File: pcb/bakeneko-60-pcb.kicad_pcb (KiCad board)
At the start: 2 copper layers, 284.8 x 106.7 mm, 149 parts, among them J1 JST SH 4-pin, SW1 Reset, U1 SRV05-4, U2 ATmega32U4-AU, Y1 16MHz

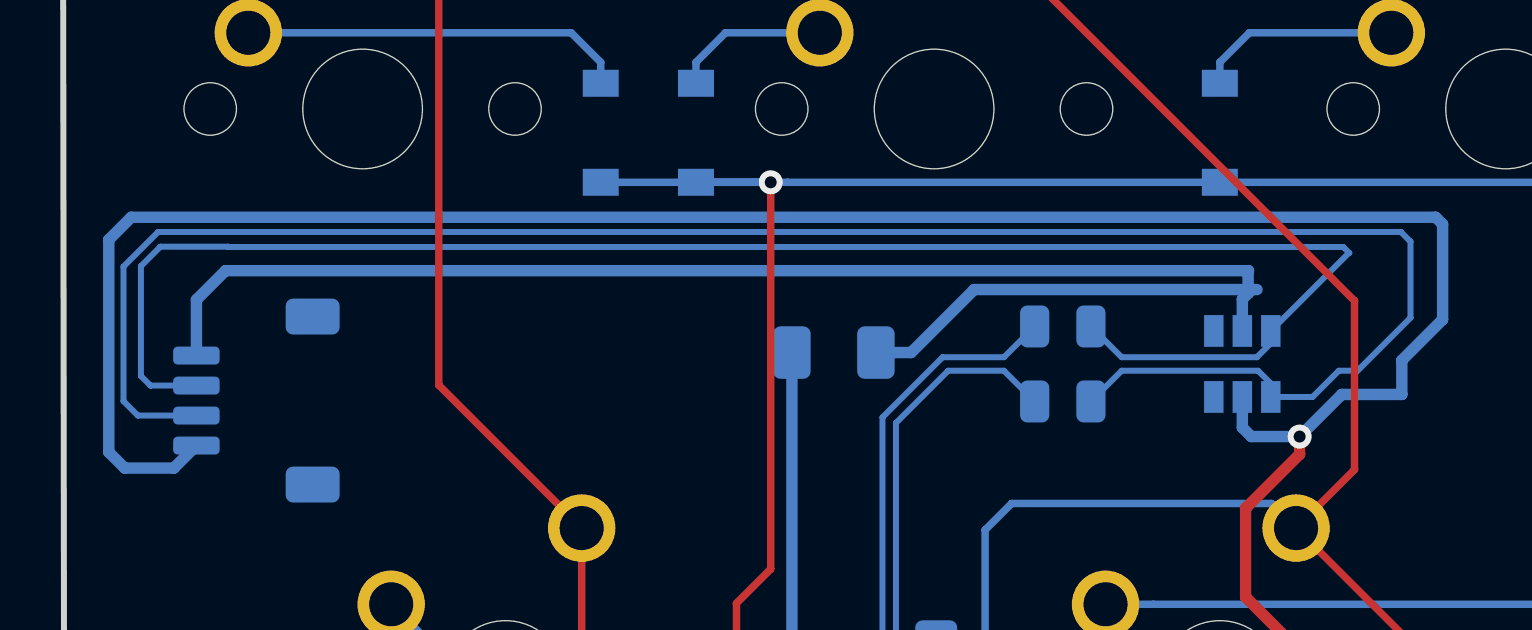
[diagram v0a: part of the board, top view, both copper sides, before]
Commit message: cleanup tracks
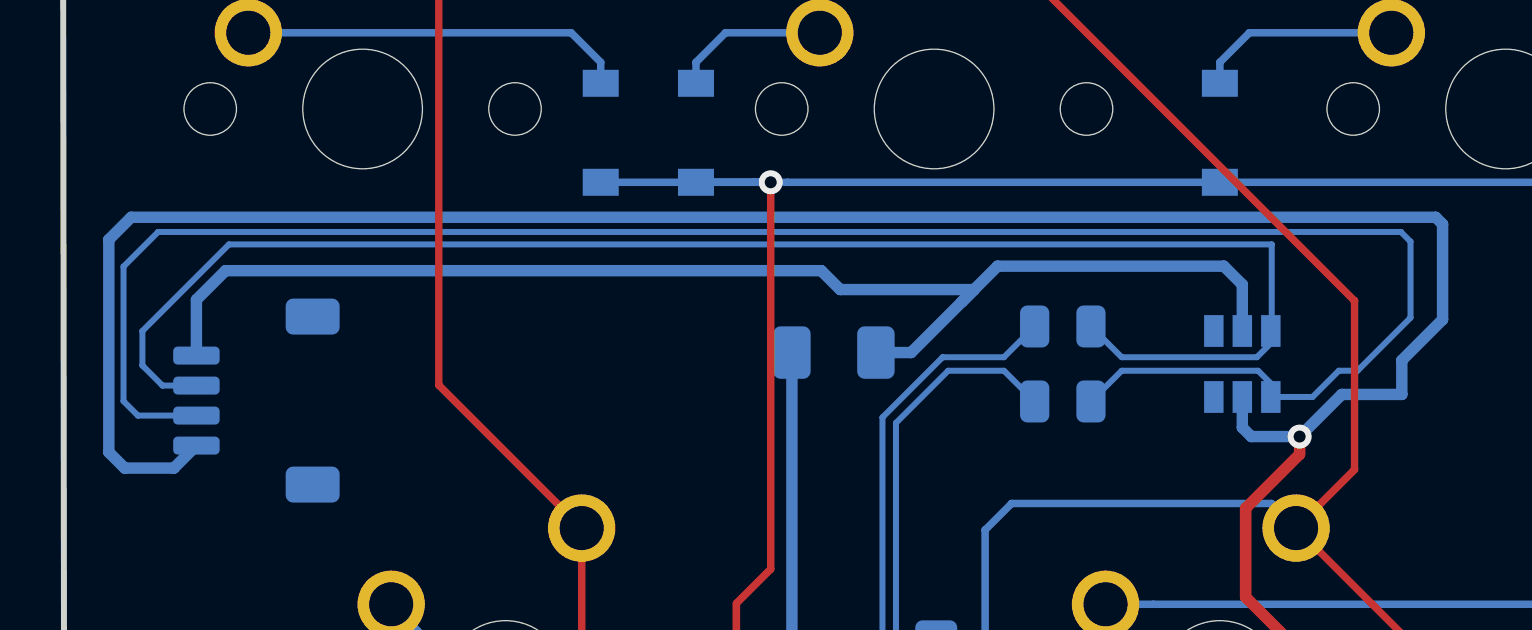
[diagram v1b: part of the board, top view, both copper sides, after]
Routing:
- net VBUS: track 53.2 -> 44.2 mm
- net D-: track 57.0 -> 52.0 mm
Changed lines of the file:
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@@
   (segment (start 262.34625 82.66) (end 261.3625 83.64375) (width 0.25) (layer "B.Cu") (net 71))
   (segment (start 267.1275 82.66) (end 262.34625 82.66) (width 0.25) (layer "B.Cu") (net 71))
-  (segment (start 38.32375 16.4) (end 38.32375 15.34) (width 0.381) (layer "B.Cu") (net 72))
-  (segment (start 38.516875 14.403125) (end 38.53 14.39) (width 0.381) (layer "B.Cu") (net 72))
-  (segment (start 38.53 14.39) (end 4.43 14.39) (width 0.381) (layer "B.Cu") (net 72))
+  (segment (start 26.11 17.12) (end 27.283694 17.12) (width 0.381) (layer "B.Cu") (net 72))
+  (segment (start 24.29 14.39) (end 4.43 14.39) (width 0.381) (layer "B.Cu") (net 72))
+  (segment (start 27.283694 17.12) (end 28.976847 15.426847) (width 0.381) (layer "B.Cu") (net 72))
+  (segment (start 38.32375 14.85375) (end 37.71 14.24) (width 0.381) (layer "B.Cu") (net 72))
+  (segment (start 28.976847 15.426847) (end 29.384311 15.019383) (width 0.381) (layer "B.Cu") (net 72))
+  (segment (start 30.163694 14.24) (end 28.976847 15.426847) (width 0.381) (layer "B.Cu") (net 72))
   (segment (start 4.43 14.39) (end 3.46 15.36) (width 0.381) (layer "B.Cu") (net 72))
-  (segment (start 38.814367 15.019383) (end 29.384311 15.019383) (width 0.381) (layer "B.Cu") (net 72))
-  (segment (start 38.516875 15.146875) (end 38.516875 14.403125) (width 0.381) (layer "B.Cu") (net 72))
-  (segment (start 27.283694 17.12) (end 26.11 17.12) (width 0.381) (layer "B.Cu") (net 72))
-  (segment (start 29.384311 15.019383) (end 27.283694 17.12) (width 0.381) (layer "B.Cu") (net 72))
+  (segment (start 37.71 14.24) (end 30.163694 14.24) (width 0.381) (layer "B.Cu") (net 72))
+  (segment (start 24.919383 15.019383) (end 24.29 14.39) (width 0.381) (layer "B.Cu") (net 72))
+  (segment (start 38.32375 16.4) (end 38.32375 14.85375) (width 0.381) (layer "B.Cu") (net 72))
+  (segment (start 29.384311 15.019383) (end 24.919383 15.019383) (width 0.381) (layer "B.Cu") (net 72))
   (segment (start 3.46 15.36) (end 3.46 17.22) (width 0.381) (layer "B.Cu") (net 72))
-  (segment (start 38.32375 15.34) (end 38.516875 15.146875) (width 0.381) (layer "B.Cu") (net 72))
-  (segment (start 38.516875 15.146875) (end 38.644367 15.019383) (width 0.381) (layer "B.Cu") (net 72))
   (segment (start 39.27375 18.15) (end 39.27375 18.6) (width 0.2) (layer "B.Cu") (net 73))
   (segment (start 39.27375 18.6) (end 40.665001 18.6) (width 0.2) (layer "B.Cu") (net 73))
@@
   (segment (start 41.540001 17.725) (end 42.165 17.725) (width 0.2) (layer "B.Cu") (net 73))
   (segment (start 1.03 18.74) (end 1.51 19.22) (width 0.2) (layer "B.Cu") (net 73))
-  (segment (start 1.93 18.22) (end 3.46 18.22) (width 0.2) (layer "B.Cu") (net 74))
-  (segment (start 41.89 13.8) (end 41.69 13.6) (width 0.2) (layer "B.Cu") (net 74))
-  (segment (start 1.61 14.24) (end 1.61 17.9) (width 0.2) (layer "B.Cu") (net 74))
-  (segment (start 4.526328 13.6) (end 4.516328 13.59) (width 0.2) (layer "B.Cu") (net 74))
-  (segment (start 41.69 13.6) (end 4.526328 13.6) (width 0.2) (layer "B.Cu") (net 74))
+  (segment (start 39.304867 13.514867) (end 4.545133 13.514867) (width 0.2) (layer "B.Cu") (net 74))
+  (segment (start 1.66 17.55) (end 2.33 18.22) (width 0.2) (layer "B.Cu") (net 74))
+  (segment (start 4.545133 13.514867) (end 1.66 16.4) (width 0.2) (layer "B.Cu") (net 74))
+  (segment (start 1.66 16.4) (end 1.66 17.55) (width 0.2) (layer "B.Cu") (net 74))
   (segment (start 34.3025 17.275) (end 38.80875 17.275) (width 0.2) (layer "B.Cu") (net 74))
-  (segment (start 39.27375 16.4) (end 41.87375 13.8) (width 0.2) (layer "B.Cu") (net 74))
-  (segment (start 2.26 13.59) (end 1.61 14.24) (width 0.2) (layer "B.Cu") (net 74))
+  (segment (start 39.304867 16.368883) (end 39.304867 13.514867) (width 0.2) (layer "B.Cu") (net 74))
   (segment (start 33.2775 16.25) (end 34.3025 17.275) (width 0.2) (layer "B.Cu") (net 74))
-  (segment (start 4.516328 13.59) (end 2.26 13.59) (width 0.2) (layer "B.Cu") (net 74))
   (segment (start 38.80875 17.275) (end 39.27375 16.81) (width 0.2) (layer "B.Cu") (net 74))
-  (segment (start 41.87375 13.8) (end 41.89 13.8) (width 0.2) (layer "B.Cu") (net 74))
-  (segment (start 1.61 17.9) (end 1.93 18.22) (width 0.2) (layer "B.Cu") (net 74))
+  (segment (start 39.27375 16.4) (end 39.304867 16.368883) (width 0.2) (layer "B.Cu") (net 74))
   (segment (start 39.27375 16.81) (end 39.27375 16.4) (width 0.2) (layer "B.Cu") (net 74))
+  (segment (start 2.33 18.22) (end 3.46 18.22) (width 0.2) (layer "B.Cu") (net 74))
   (segment (start 23.44625 61.07) (end 24.643741 59.872509) (width 0.25) (layer "F.Cu") (net 78))
   (segment (start 24.643741 59.872509) (end 24.643741 51.179221) (width 0.25) (layer "F.Cu") (net 78))
